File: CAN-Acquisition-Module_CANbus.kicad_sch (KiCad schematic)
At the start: 20 parts, among them J5 OSTVN04A150, J6 OSTVN04A150, U5 SN65HVD234

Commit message: BOM updated for LCSC. Still a WIP.
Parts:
- C33, C38, C39, R17, R18, R19, R21, R22, R23, R24: LCSC (none) -> DNP
- J5, J6: LCSC (none) -> C708735; Mfr. On Shore Technology -> On-Shore
- R20, R25: Tolerance (none) -> 1%
- U5: LCSC (none) -> C111810
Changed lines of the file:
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@@
     )
     (property "Do Not Place" "DNP" (id 4) (at 219.71 123.19 90))
+    (property "LCSC" "DNP" (id 5) (at 215.9 119.38 0)
+      (effects (font (size 1.27 1.27)) hide)
+    )
     (pin "1")
     (pin "2")
@@
     )
     (property "Do Not Place" "DNP" (id 4) (at 198.12 115.57 0))
+    (property "LCSC" "DNP" (id 5) (at 194.31 111.76 0)
+      (effects (font (size 1.27 1.27)) hide)
+    )
     (pin "1")
     (pin "2")
@@
     )
     (property "Do Not Place" "DNP" (id 4) (at 218.44 93.98 0))
+    (property "LCSC" "DNP" (id 5) (at 214.63 97.79 0)
+      (effects (font (size 1.27 1.27)) hide)
+    )
     (pin "1")
     (pin "2")
@@
     )
     (property "Do Not Place" "DNP" (id 4) (at 100.33 93.98 0))
+    (property "LCSC" "DNP" (id 5) (at 97.79 91.44 0)
+      (effects (font (size 1.27 1.27)) hide)
+    )
     (pin "1")
     (pin "2")
@@
       (effects (font (size 1.27 1.27)) hide)
     )
-    (property "Mfr." "On Shore Technology" (id 5) (at 66.04 67.31 0)
+    (property "Mfr." "On-Shore" (id 5) (at 66.04 67.31 0)
+      (effects (font (size 1.27 1.27)) hide)
+    )
+    (property "LCSC" "C708735" (id 6) (at 66.04 67.31 0)
       (effects (font (size 1.27 1.27)) hide)
     )
@@
       (effects (font (size 1.27 1.27)) hide)
     )
+    (property "Tolerance" "1%" (id 6) (at 243.84 97.79 0)
+      (effects (font (size 1.27 1.27)) hide)
+    )
     (pin "1")
     (pin "2")
@@
     )
     (property "Do Not Place" "DNP" (id 4) (at 237.49 106.68 0))
+    (property "LCSC" "DNP" (id 5) (at 233.68 102.87 0)
+      (effects (font (size 1.27 1.27)) hide)
+    )
     (pin "1")
     (pin "2")
@@
     )
     (property "Do Not Place" "DNP" (id 4) (at 213.36 128.27 0))
+    (property "LCSC" "DNP" (id 5) (at 208.28 124.46 0)
+      (effects (font (size 1.27 1.27)) hide)
+    )
     (pin "1")
     (pin "2")
@@
     )
     (property "Datasheet" "http://www.ti.com/lit/ds/symlink/sn65hvd234.pdf" (id 3) (at 176.53 72.39 0)
+      (effects (font (size 1.27 1.27)) hide)
+    )
+    (property "LCSC" "C111810" (id 4) (at 173.99 82.55 0)
       (effects (font (size 1.27 1.27)) hide)
     )
@@
       (effects (font (size 1.27 1.27)) hide)
     )
+    (property "LCSC" "DNP" (id 5) (at 101.6 105.41 0)
+      (effects (font (size 1.27 1.27)) hide)
+    )
     (pin "1")
     (pin "2")
@@
     )
     (property "Do Not Place" "DNP" (id 4) (at 227.33 96.52 0))
+    (property "LCSC" "DNP" (id 5) (at 223.52 92.71 0)
+      (effects (font (size 1.27 1.27)) hide)
+    )
     (pin "1")
     (pin "2")
@@
     )
     (property "Do Not Place" "DNP" (id 4) (at 227.33 105.41 0))
+    (property "LCSC" "DNP" (id 5) (at 223.52 101.6 0)
+      (effects (font (size 1.27 1.27)) hide)
+    )
     (pin "1")
     (pin "2")
@@
       (effects (font (size 1.27 1.27)) hide)
     )
-    (property "Mfr." "On Shore Technology" (id 5) (at 36.83 64.77 0)
+    (property "Mfr." "On-Shore" (id 5) (at 36.83 64.77 0)
+      (effects (font (size 1.27 1.27)) hide)
+    )
+    (property "LCSC" "C708735" (id 6) (at 36.83 64.77 0)
       (effects (font (size 1.27 1.27)) hide)
     )
@@
       (effects (font (size 1.27 1.27)) hide)
     )
+    (property "Tolerance" "1%" (id 6) (at 194.31 123.19 0)
+      (effects (font (size 1.27 1.27)) hide)
+    )
     (pin "1")
     (pin "2")
@@
     )
     (property "Do Not Place" "DNP" (id 4) (at 109.22 93.98 0))
-    (pin "1")
-    (pin "2")
+    (property "LCSC" "DNP" (id 5) (at 106.68 91.44 0)
+      (effects (font (size 1.27 1.27)) hide)
+    )
+    (pin "1")
+    (pin "2")

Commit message: BOM updated for LCSC. Still a WIP
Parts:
- D10: LCSC (none) -> C284078
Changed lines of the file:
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@@
+      (effects (font (size 1.27 1.27)) hide)
+    )
+    (property "LCSC" "C284078" (id 6) (at 67.31 92.71 0)
       (effects (font (size 1.27 1.27)) hide)
     )

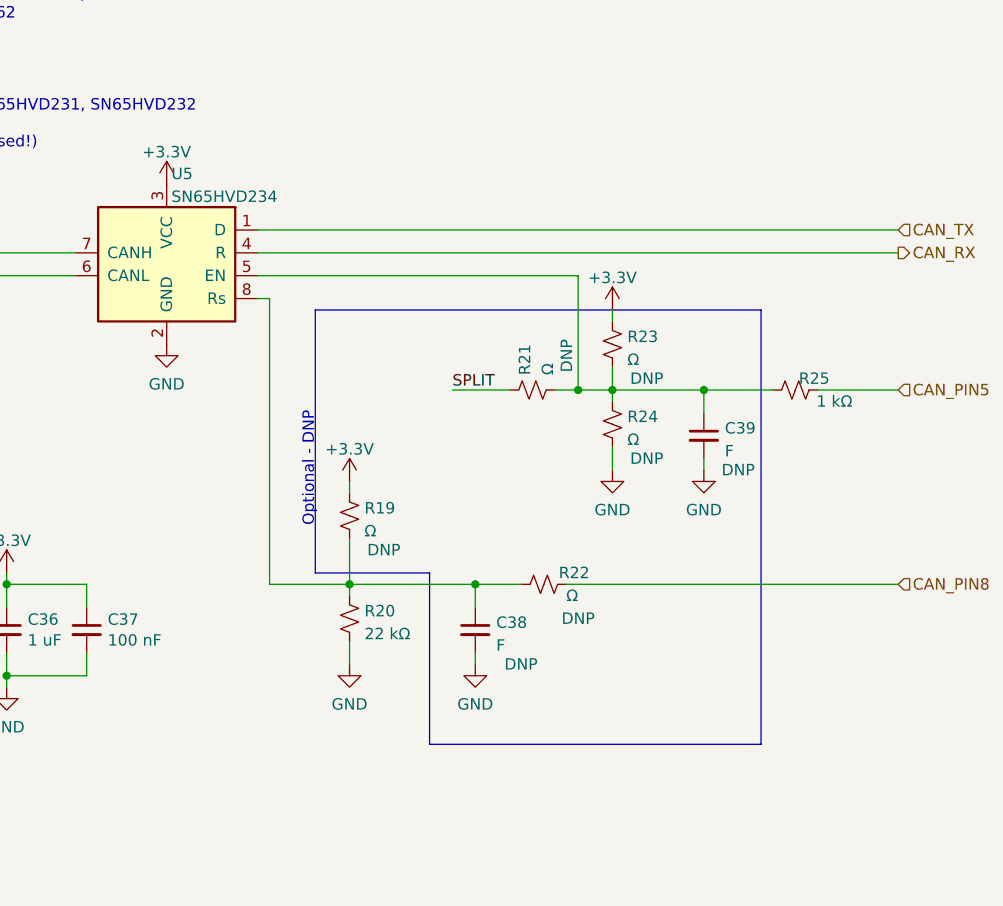
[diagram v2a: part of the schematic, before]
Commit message: Added differential BOM for order (to be removed later)
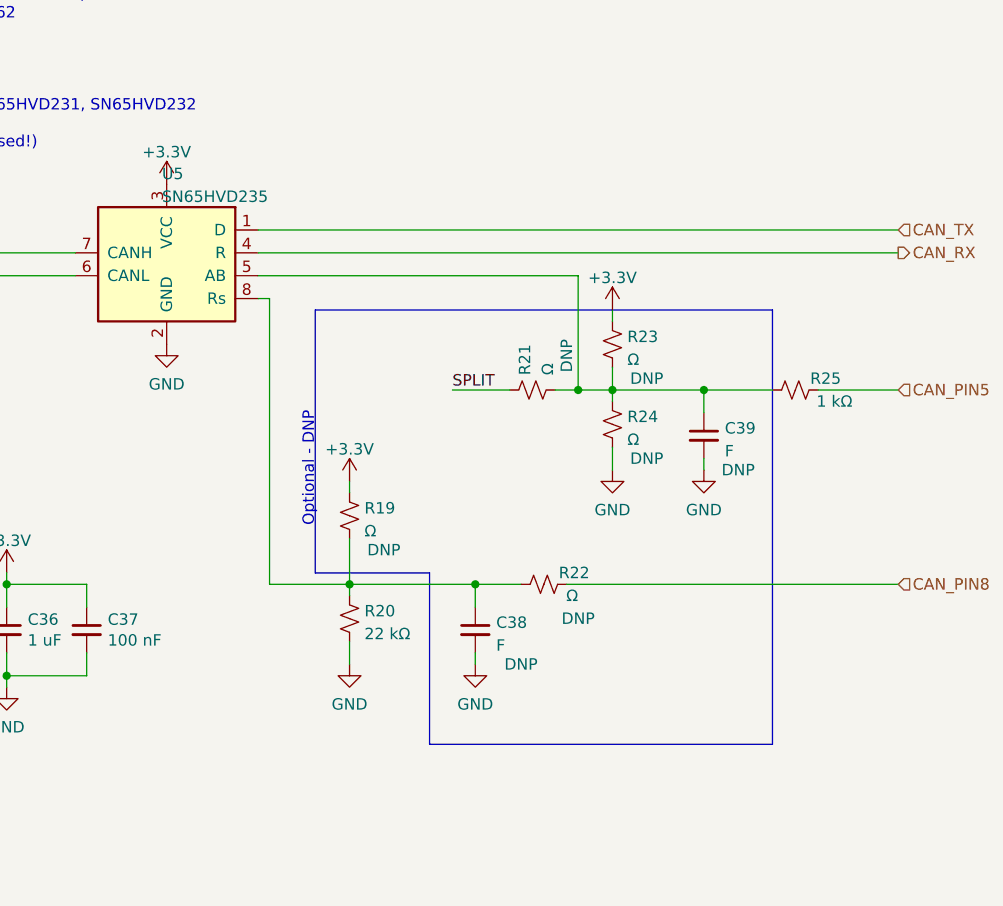
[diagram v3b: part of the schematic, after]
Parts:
- U5: value SN65HVD234 -> SN65HVD235
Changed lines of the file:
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@@
     (stroke (width 0) (type default) (color 0 0 0 0))
   )
-  (polyline (pts (xy 203.2 137.16) (xy 240.03 137.16))
+  (polyline (pts (xy 203.2 137.16) (xy 241.3 137.16))
     (stroke (width 0) (type default) (color 0 0 0 0))
   )
@@
     (stroke (width 0) (type default) (color 0 0 0 0))
   )
-  (polyline (pts (xy 240.03 137.16) (xy 240.03 88.9))
+  (polyline (pts (xy 241.3 137.16) (xy 241.3 88.9))
     (stroke (width 0) (type default) (color 0 0 0 0))
   )
@@
     (stroke (width 0) (type default) (color 0 0 0 0))
   )
-  (polyline (pts (xy 240.03 88.9) (xy 190.5 88.9))
+  (polyline (pts (xy 241.3 88.9) (xy 190.5 88.9))
     (stroke (width 0) (type default) (color 0 0 0 0))
   )
@@
   (symbol (lib_id "Device:R_Small_US") (at 243.84 97.79 90) (unit 1)
     (in_bom yes) (on_board yes)
-    (property "Reference" "R25" (id 0) (at 247.65 96.52 90)
+    (property "Reference" "R25" (id 0) (at 248.92 96.52 90)
       (effects (font (size 1.27 1.27)) (justify left))
     )
@@
     )
     (property "Tolerance" "1%" (id 6) (at 243.84 97.79 0)
+      (effects (font (size 1.27 1.27)) hide)
+    )
+    (property "Do Not Place" "" (id 7) (at 247.65 101.6 90)
       (effects (font (size 1.27 1.27)) hide)
     )
@@
   (symbol (lib_id "Interface_CAN_LIN:SN65HVD234") (at 173.99 82.55 0) (mirror y) (unit 1)
     (in_bom yes) (on_board yes) (fields_autoplaced)
-    (property "Reference" "U5" (id 0) (at 174.5106 73.7702 0)
+    (property "Reference" "U5" (id 0) (at 173.4694 73.7702 0)
       (effects (font (size 1.27 1.27)) (justify right))
     )
-    (property "Value" "SN65HVD234" (id 1) (at 174.5106 76.3071 0)
+    (property "Value" "SN65HVD235" (id 1) (at 173.4694 76.3071 0)
       (effects (font (size 1.27 1.27)) (justify right))
     )
@@
       (effects (font (size 1.27 1.27)) hide)
     )
-    (property "Datasheet" "http://www.ti.com/lit/ds/symlink/sn65hvd234.pdf" (id 3) (at 176.53 72.39 0)
-      (effects (font (size 1.27 1.27)) hide)
-    )
+    (property "Datasheet" "http://www.ti.com/lit/ds/symlink/sn65hvd234.pdf" (id 3) (at 171.45 72.39 0)
+      (effects (font (size 1.27 1.27)) hide)
+    )
